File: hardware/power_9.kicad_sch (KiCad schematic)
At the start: 20 parts, among them J11 TBC 2.54mm 10A, U8 AP63203WU, U9 XC6206P182MR

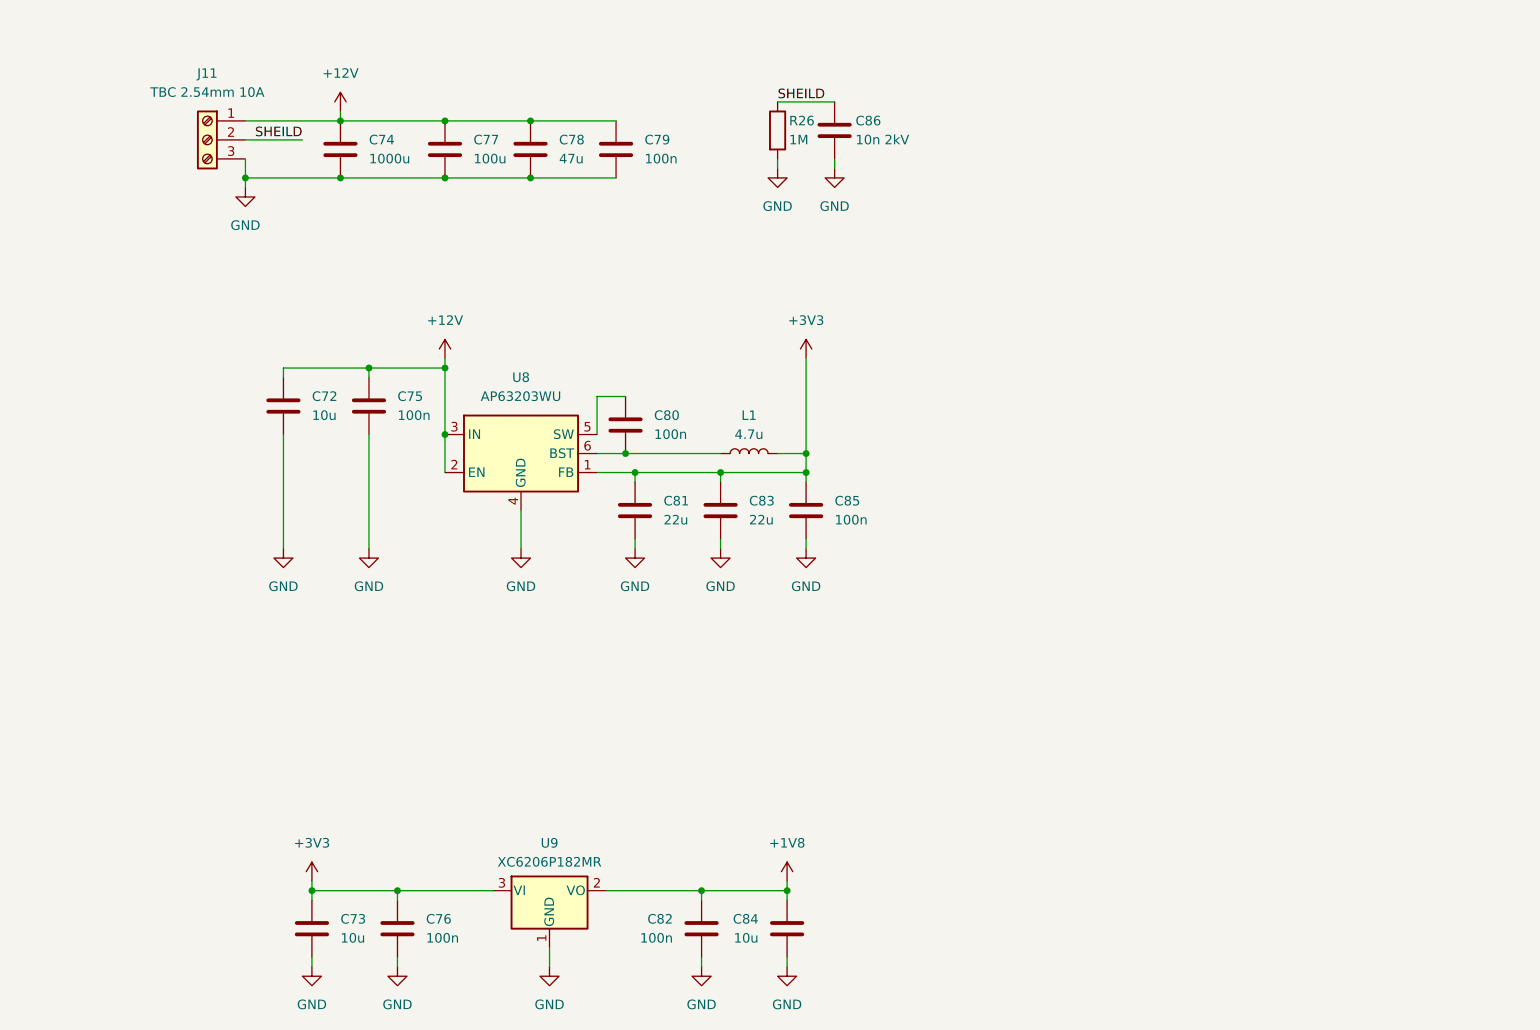
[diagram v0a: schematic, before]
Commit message: Organize schematic
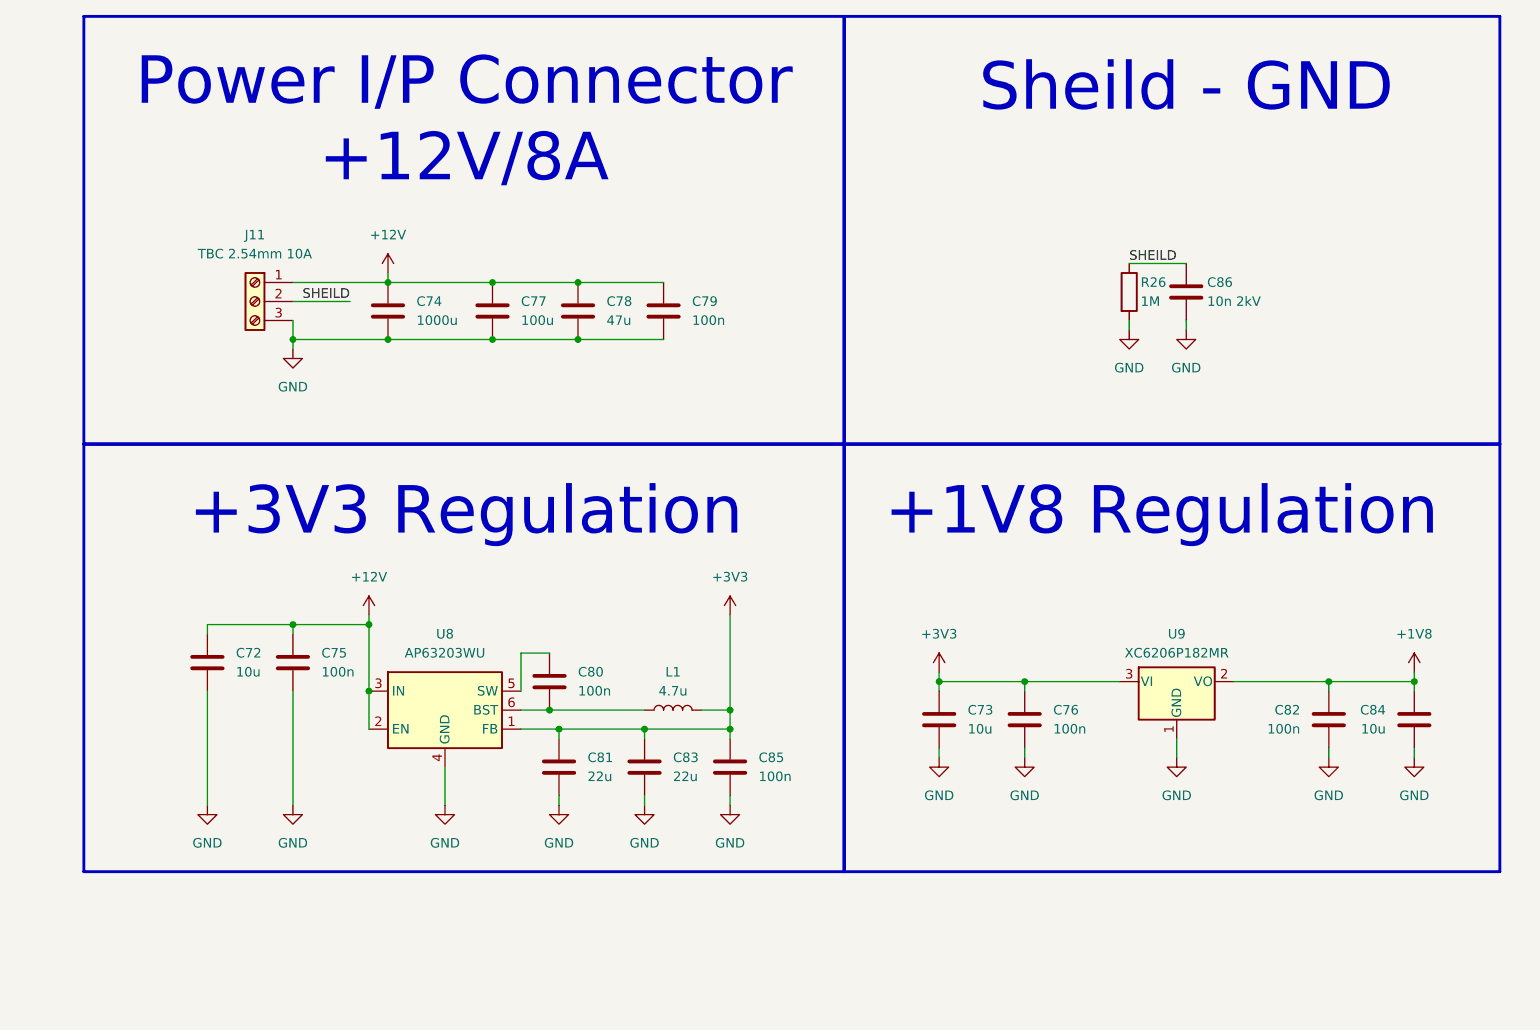
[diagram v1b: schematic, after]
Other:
- note added: "+1V8 Regulation"
- note added: "+3V3 Regulation"
- note added: "Power I/P Connector +12V/8A"
- note added: "Sheild - GND"
- moved on the sheet: C72, C73, C74, C75, C76, C77, C78, C79, C80, C81, C82, C83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

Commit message: Link footprints to Symbols
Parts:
- C72, C73, C75, C76, C80, C81, C82, C83, C84, C85: footprint Package_TO_SOT_SMD:TSOT-23-6 -> STM32F407 Dev Kit Library:C_0805_2012Metric_Pad1.18x1.45mm_HandSolder
- C74, C77, C78, C79: footprint (none) -> STM32F407 Dev Kit Library:C_0805_2012Metric_Pad1.18x1.45mm_HandSolder
- C86: footprint Package_QFP:LQFP-48_7x7mm_P0.5mm -> STM32F407 Dev Kit Library:C_1812_4532Metric_Pad1.57x3.40mm_HandSolder
- J11: footprint (none) -> STM32F407 Dev Kit Library:TerminalBlock_Xinya_XY308-2.54-3P_1x03_P2.54mm_Horizontal
- L1: footprint (none) -> STM32F407 Dev Kit Library:L_0805_2012Metric_Pad1.05x1.20mm_HandSolder
- R26: footprint (none) -> STM32F407 Dev Kit Library:R_0805_2012Metric_Pad1.20x1.40mm_HandSolder
- U8: footprint Package_TO_SOT_SMD:TSOT-23-6 -> STM32F407 Dev Kit Library:TSOT-23-6_HandSoldering
- U9: footprint Package_TO_SOT_SMD:SOT-23-3 -> STM32F407 Dev Kit Library:SOT-23-3
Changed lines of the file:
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@@
 			)
 		)
-		(property "Footprint" "Package_TO_SOT_SMD:TSOT-23-6"
+		(property "Footprint" "STM32F407 Dev Kit Library:C_0805_2012Metric_Pad1.18x1.45mm_HandSolder"
 			(at 216.2048 129.54 0)
 			(hide yes)
@@
 			)
 		)
-		(property "Footprint" "Package_TO_SOT_SMD:TSOT-23-6"
+		(property "Footprint" "STM32F407 Dev Kit Library:C_0805_2012Metric_Pad1.18x1.45mm_HandSolder"
 			(at 68.2752 121.92 0)
 			(hide yes)
@@
 			)
 		)
-		(property "Footprint" ""
+		(property "Footprint" "STM32F407 Dev Kit Library:C_0805_2012Metric_Pad1.18x1.45mm_HandSolder"
 			(at 92.4052 74.93 0)
 			(hide yes)
@@
 			)
 		)
-		(property "Footprint" ""
+		(property "Footprint" "STM32F407 Dev Kit Library:C_0805_2012Metric_Pad1.18x1.45mm_HandSolder"
 			(at 117.8052 74.93 0)
 			(hide yes)
@@
 			)
 		)
-		(property "Footprint" "Package_QFP:LQFP-48_7x7mm_P0.5mm"
+		(property "Footprint" "STM32F407 Dev Kit Library:C_1812_4532Metric_Pad1.57x3.40mm_HandSolder"
 			(at 199.0852 72.39 0)
 			(hide yes)
@@
 			)
 		)
-		(property "Footprint" ""
+		(property "Footprint" "STM32F407 Dev Kit Library:C_0805_2012Metric_Pad1.18x1.45mm_HandSolder"
 			(at 129.2352 74.93 0)
 			(hide yes)
@@
 			)
 		)
-		(property "Footprint" "Package_TO_SOT_SMD:TSOT-23-6"
+		(property "Footprint" "STM32F407 Dev Kit Library:C_0805_2012Metric_Pad1.18x1.45mm_HandSolder"
 			(at 227.6348 129.54 0)
 			(hide yes)
@@
 			)
 		)
-		(property "Footprint" "Package_TO_SOT_SMD:TSOT-23-6"
+		(property "Footprint" "STM32F407 Dev Kit Library:C_0805_2012Metric_Pad1.18x1.45mm_HandSolder"
 			(at 115.2652 135.89 0)
 			(hide yes)
@@
 			)
 		)
-		(property "Footprint" ""
+		(property "Footprint" "STM32F407 Dev Kit Library:C_0805_2012Metric_Pad1.18x1.45mm_HandSolder"
 			(at 106.3752 74.93 0)
 			(hide yes)
@@
 			)
 		)
-		(property "Footprint" "Package_TO_SOT_SMD:TSOT-23-6"
+		(property "Footprint" "STM32F407 Dev Kit Library:C_0805_2012Metric_Pad1.18x1.45mm_HandSolder"
 			(at 126.6952 135.89 0)
 			(hide yes)
@@
 			)
 		)
-		(property "Footprint" "Package_TO_SOT_SMD:TSOT-23-6"
+		(property "Footprint" "STM32F407 Dev Kit Library:C_0805_2012Metric_Pad1.18x1.45mm_HandSolder"
 			(at 138.1252 135.89 0)
 			(hide yes)
@@
 			)
 		)
-		(property "Footprint" "Package_TO_SOT_SMD:TSOT-23-6"
+		(property "Footprint" "STM32F407 Dev Kit Library:TSOT-23-6_HandSoldering"
 			(at 99.06 147.32 0)
 			(hide yes)
@@
 			)
 		)
-		(property "Footprint" "Package_TO_SOT_SMD:TSOT-23-6"
+		(property "Footprint" "STM32F407 Dev Kit Library:C_0805_2012Metric_Pad1.18x1.45mm_HandSolder"
 			(at 177.4952 129.54 0)
 			(hide yes)
@@
 			)
 		)
-		(property "Footprint" ""
+		(property "Footprint" "STM32F407 Dev Kit Library:L_0805_2012Metric_Pad1.05x1.20mm_HandSolder"
 			(at 129.54 124.46 0)
 			(hide yes)
@@
 			)
 		)
-		(property "Footprint" ""
+		(property "Footprint" "STM32F407 Dev Kit Library:R_0805_2012Metric_Pad1.20x1.40mm_HandSolder"
 			(at 188.722 68.58 90)
 			(hide yes)
@@
 			)
 		)
-		(property "Footprint" "Package_TO_SOT_SMD:SOT-23-3"
+		(property "Footprint" "STM32F407 Dev Kit Library:SOT-23-3"
 			(at 196.85 114.935 0)
 			(hide yes)
@@
 			)
 		)
-		(property "Footprint" "Package_TO_SOT_SMD:TSOT-23-6"
+		(property "Footprint" "STM32F407 Dev Kit Library:C_0805_2012Metric_Pad1.18x1.45mm_HandSolder"
 			(at 113.9952 124.46 0)
 			(hide yes)
@@
 			)
 		)
-		(property "Footprint" "Package_TO_SOT_SMD:TSOT-23-6"
+		(property "Footprint" "STM32F407 Dev Kit Library:C_0805_2012Metric_Pad1.18x1.45mm_HandSolder"
 			(at 79.7052 121.92 0)
 			(hide yes)
@@
 			)
 		)
-		(property "Footprint" ""
+		(property "Footprint" "STM32F407 Dev Kit Library:TerminalBlock_Xinya_XY308-2.54-3P_1x03_P2.54mm_Horizontal"
 			(at 73.66 69.85 0)
 			(hide yes)
@@
 			)
 		)
-		(property "Footprint" "Package_TO_SOT_SMD:TSOT-23-6"
+		(property "Footprint" "STM32F407 Dev Kit Library:C_0805_2012Metric_Pad1.18x1.45mm_HandSolder"
 			(at 166.0652 129.54 0)
 			(hide yes)
